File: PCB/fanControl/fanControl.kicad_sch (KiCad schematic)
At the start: 81 parts, among them J1 USB_B_Micro, J2 Barrel_Jack_Switch, J3 Conn_01x03, J4 Conn_01x06, J5 Conn_01x04, Q1 PNM723, Q2 FDD4243, Q3 BC547, Q4 PNM723, Q5 BC847BDW1, Q6 SI2324A, U1 DS18B20, U2 CH340B, U3 LM2575BT-ADJ, U4 ESP-12E, U5 LD1117S33CTR, Y1 12M

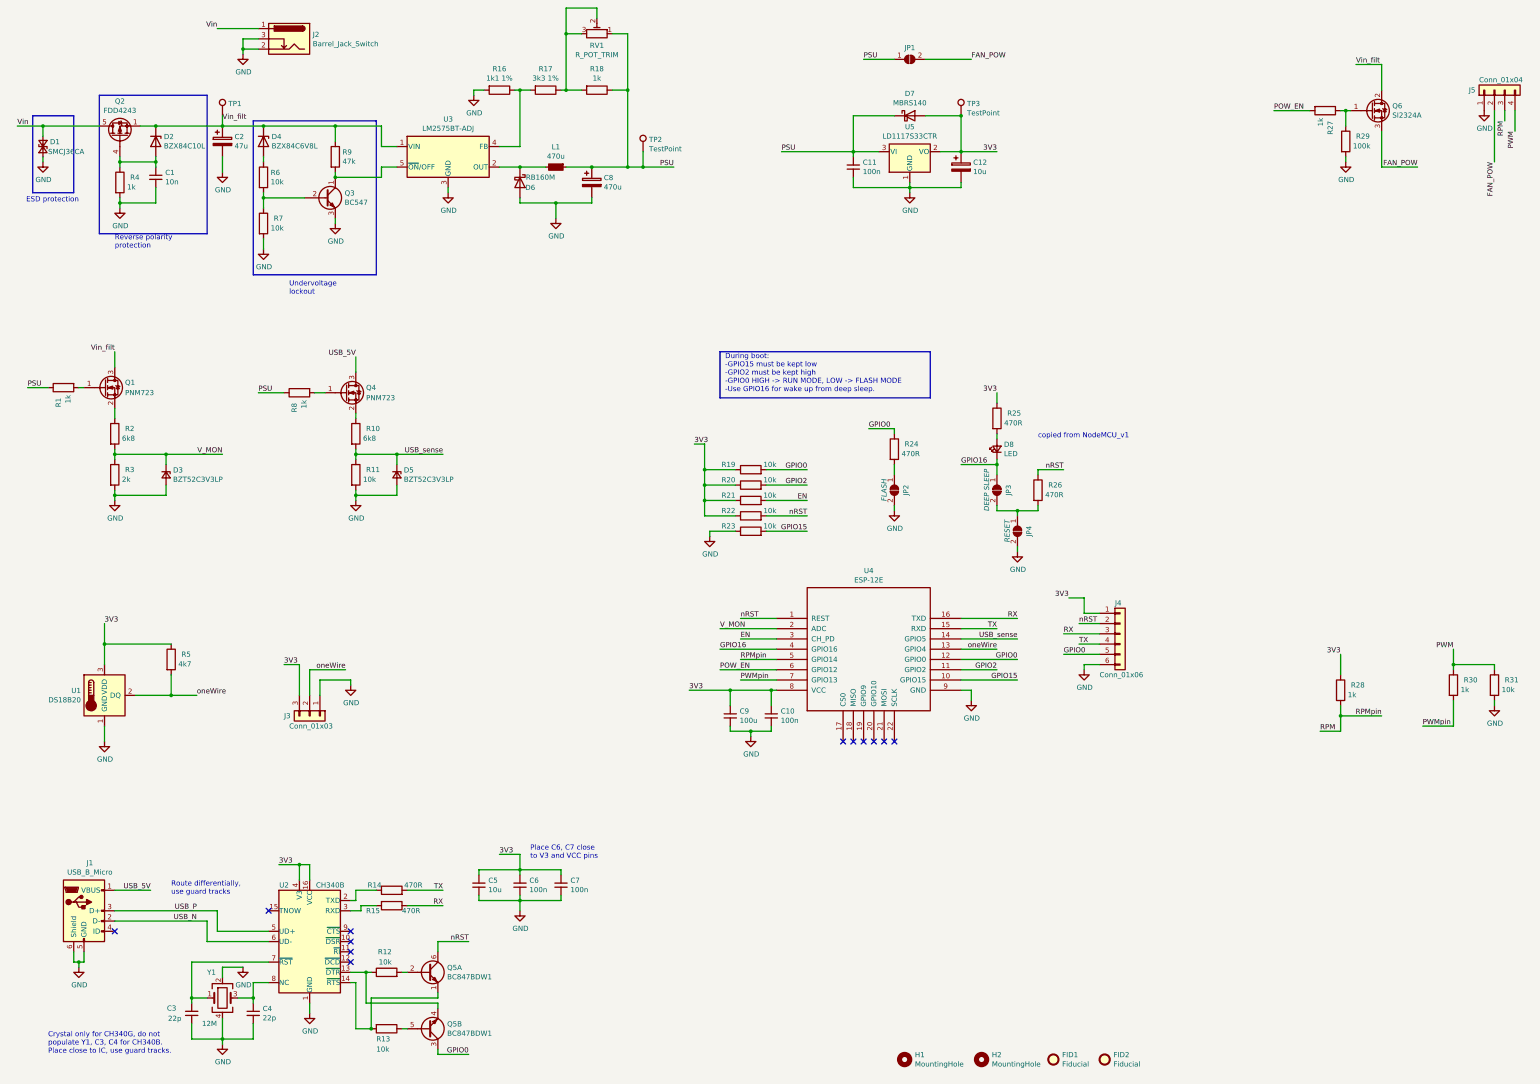
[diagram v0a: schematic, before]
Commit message: LCSC BOM done
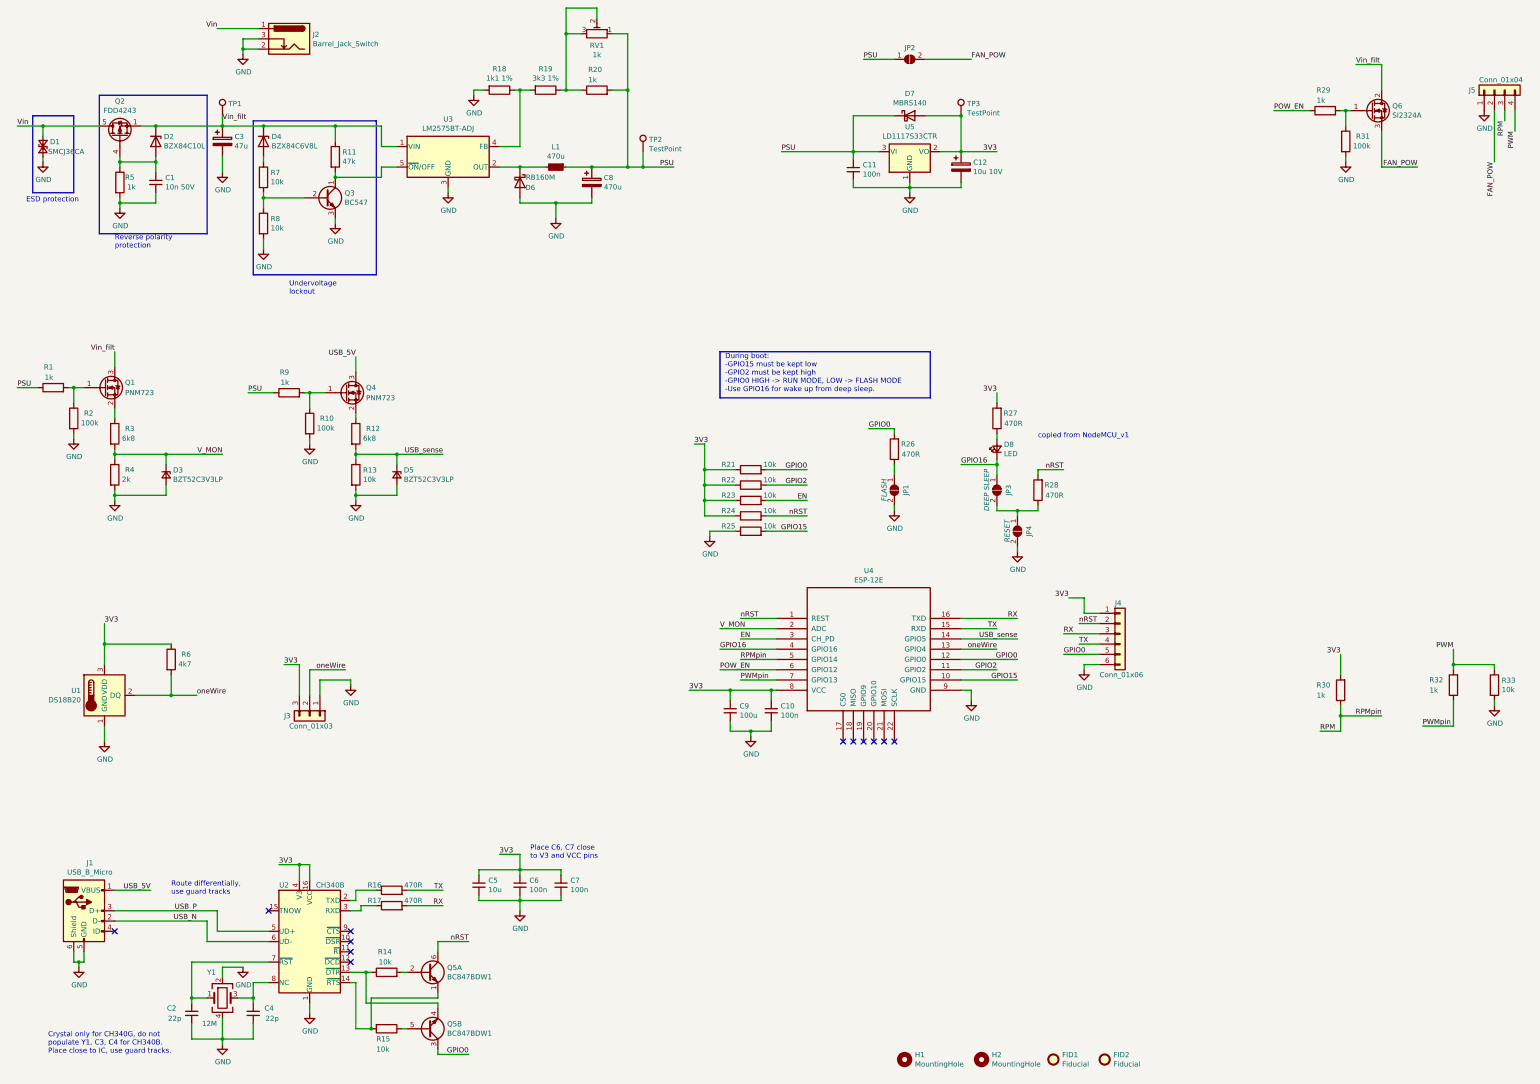
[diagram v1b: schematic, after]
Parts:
- removed R11, R19, R31, R7: 10k, agro-footprint:RES_0805, symbol Device:R
- removed R18: 1k, agro-footprint:RES_0805, symbol Device:R
- added R14, R33: 10k, agro-footprint:RES_0805, symbol Device:R
- added R17: 470R, agro-footprint:RES_0805, symbol Device:R
- added R2: 100k, agro-footprint:RES_0805, symbol Device:R
- added R29, R32, R9: 1k, agro-footprint:RES_0805, symbol Device:R
- C1: value 10n -> 10n 50V; LCSC (none) -> C527201; MPN (none) -> CC0805JKNPO9BN103; Manufacturer (none) -> Yageo
- C10, C11, C6, C7: LCSC (none) -> C520058; MPN (none) -> CC0805GRNPO9BN220; Manufacturer (none) -> Yageo
- C12: value 10u -> 10u 10V; LCSC (none) -> C696821; MPN (none) -> T529P106M010AAE200; Manufacturer Vishay -> KEMET; PartNo 293D106X9016A2TE3 -> (none)
- C2: renamed from C3; LCSC (none) -> C541515; MPN (none) -> CC0805FRNPO9BN220; Manufacturer (none) -> Yageo
- C4: LCSC (none) -> C541515; MPN (none) -> CC0805FRNPO9BN220; Manufacturer (none) -> Yageo
- C5: LCSC (none) -> C88484; MPN (none) -> CC0805ZKY5V6BB106; Manufacturer (none) -> Yageo
- C9: footprint agro-footprint:CAP_0805 -> Capacitor_SMD:C_1206_3216Metric; LCSC (none) -> C110048; MPN (none) -> CC1206MKX5R5BB107; Manufacturer (none) -> Yageo
- D2: Field6 BZX84C10LT1G -> (none); MPN (none) -> BZX84C10LT1G
- D8: LCSC (none) -> C131208; MPN (none) -> 17-215/BHC-AP1Q2/3T; Manufacturer (none) -> Everlight Elec
- J3, J4, J5, JP3, JP4, TP1, TP2, TP3: now left out of the parts list
- JP1: renamed from JP2; now left out of the parts list
- JP2: renamed from JP1; now left out of the parts list
- R1, R30: LCSC (none) -> C100046; MPN (none) -> RC0805JR-071KL; Manufacturer (none) -> Yageo
- R10: value 6k8 -> 100k; LCSC (none) -> C100049; MPN (none) -> RC0805JR-07100KL; Manufacturer (none) -> Yageo
- R11: renamed from R9; LCSC (none) -> C131051; MPN (none) -> RC0805JR-0747KL; Manufacturer (none) -> Yageo
- R12: value 10k -> 6k8; LCSC (none) -> C137409; MPN (none) -> RC0805JR-076K8L; Manufacturer (none) -> Yageo
- R13, R21, R22, R23: LCSC (none) -> C100047; MPN (none) -> RC0805JR-0710KL; Manufacturer (none) -> Yageo
- R15, R24, R25: value 470R -> 10k; LCSC (none) -> C100047; MPN (none) -> RC0805JR-0710KL; Manufacturer (none) -> Yageo
- R16: renamed from R14; LCSC (none) -> C114747; MPN (none) -> RC0805JR-07470RL; Manufacturer (none) -> Yageo
- R18: renamed from R16; LCSC (none) -> C185294; MPN (none) -> RC0805FR-071K1L; Manufacturer (none) -> Yageo
- R19: renamed from R17; LCSC (none) -> C114531; MPN (none) -> RC0805FR-073K3L; Manufacturer (none) -> Yageo
- R20: value 10k -> 1k; LCSC (none) -> C100046; MPN (none) -> RC0805JR-071KL; Manufacturer (none) -> Yageo
- R26: LCSC (none) -> C114747; MPN (none) -> RC0805JR-07470RL; Manufacturer (none) -> Yageo
- R27, R28: value 1k -> 470R; LCSC (none) -> C114747; MPN (none) -> RC0805JR-07470RL; Manufacturer (none) -> Yageo
- R3: renamed from R2; LCSC (none) -> C137409; MPN (none) -> RC0805JR-076K8L; Manufacturer (none) -> Yageo
- R31: renamed from R29; LCSC (none) -> C100049; MPN (none) -> RC0805JR-07100KL; Manufacturer (none) -> Yageo
- R4: renamed from R3; LCSC (none) -> C114748; MPN (none) -> RC0805JR-072KL; Manufacturer (none) -> Yageo
- R5: renamed from R4; LCSC (none) -> C100046; MPN (none) -> RC0805JR-071KL; Manufacturer (none) -> Yageo
- R6: renamed from R5; LCSC (none) -> C105427; MPN (none) -> RC0805JR-074K7L; Manufacturer (none) -> Yageo
- R7: renamed from R6; LCSC (none) -> C100047; MPN (none) -> RC0805JR-0710KL; Manufacturer (none) -> Yageo
- R8: value 1k -> 10k; LCSC (none) -> C100047; MPN (none) -> RC0805JR-0710KL; Manufacturer (none) -> Yageo
- RV1: value R_POT_TRIM -> 1k
- renumbered C2 to C3
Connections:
- net 3V3: now also R23.1, R24.1, R27.2, R30.2; no longer R20.1, R25.1, R28.1
- net EN: now also R23.2; no longer R21.2
- net GND: now also C4.1, R10.2, R13.2, R25.1, R8.2, R2.2, R33.2; no longer C4.2, R23.1
- net GPIO0: now also R21.2, R26.2; no longer R24.1
- net GPIO15: now also R25.2; no longer R23.2
- net GPIO2: now also R22.2; no longer R20.2
- net POW_EN: now also R29.1; no longer R27.2
- net PSU: now also R20.2, R9.1; no longer R8.1
- net PWM: now also R32.2, R33.1; no longer R30.1
- net PWMpin: now also R32.1; no longer R30.2
- net RPM: now also R30.1; no longer R28.2
- net RX: now also R17.2; no longer R15.1
- net USB_sense: now also R12.2, R13.1; no longer R10.2
- net nRST: now also R24.2, R28.2; no longer R22.2, R26.1
- net at Q3.2 (B), R7.2: now also R8.1
- net at R19.1, RV1.2, RV1.3: now also R20.1
- net at Q6.1 (G), R31.1: now also R29.2; no longer R27.1
- net at R10.1: now also Q4.1 (G), R9.2; no longer Q4.2 (S)
- net at Q1.1 (G), R1.2: now also R2.1
- net at R15.2: now also Q5.1 (E1), U2.14 (~{RTS}); no longer U2.3 (RXD)
- net at U2.8 (NC), Y1.3: now also C4.2; no longer C4.1
- net at Q5.5 (B2): now also R15.1; no longer R13.1
- net at Q5.4 (E2), U2.13 (~{DTR}): now also R14.1; no longer R12.1
- net at Q5.2 (B1): now also R14.2; no longer R12.2
- net at JP1.1 (A): now also R26.1; no longer R24.2
- net at D8.2 (A): now also R27.1; no longer R25.2
- net at JP3.2 (B), JP4.1 (A): now also R28.1; no longer R26.2
- new net: R17.1, U2.3 (RXD)
- new net: Q4.2 (S), R12.1
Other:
- moved on the sheet: C1, C9

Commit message: ver2
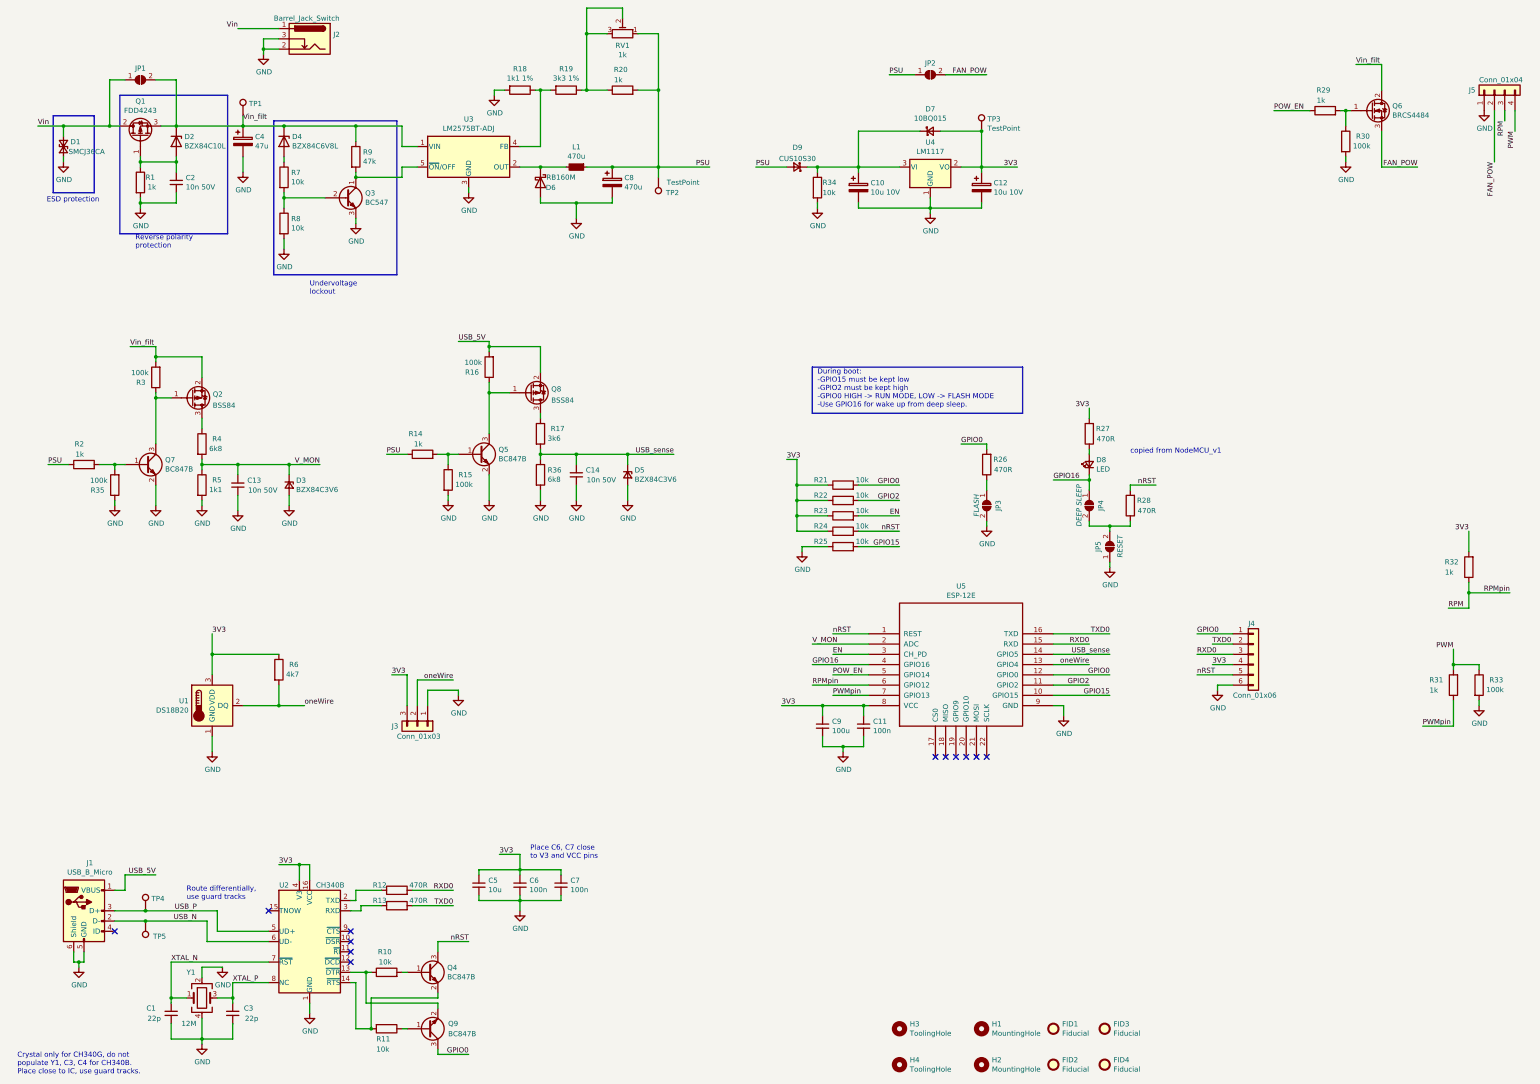
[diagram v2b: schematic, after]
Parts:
- removed C11: 100n, agro-footprint:CAP_0805, symbol agro-symbol:CAP
- removed Q1, Q4: PNM723, Package_TO_SOT_SMD:SOT-723, symbol Device:Q_NMOS_GSD
- removed Q2: FDD4243, fanControl:TO-252-2_TabPin5, symbol Transistor_FET:DMP3013SFV
- removed Q5: BC847BDW1, Package_TO_SOT_SMD:SOT-363_SC-70-6, symbol Transistor_BJT:BC847BDW1
- removed R12: 6k8, agro-footprint:RES_0805, symbol Device:R
- removed R13: 10k, agro-footprint:RES_0805, symbol Device:R
- added C10: 10u 10V, Capacitor_Tantalum_SMD:CP_EIA-3216-18_Kemet-A_Pad1.58x1.35mm_HandSolder, symbol Device:CP
- added C13, C14: 10n 50V, agro-footprint:CAP_0805, symbol agro-symbol:CAP
- added D9: CUS10S30, Diode_SMD:D_SOD-323_HandSoldering, symbol agro-symbol:SCHOTTKY
- added FID2, FID4: Fiducial, Fiducial:Fiducial_0.5mm_Mask1.5mm, symbol Mechanical:Fiducial
- added H3, H4: ToolingHole, fanControl:JLC_toolinghole, symbol Mechanical:MountingHole
- added JP1: SolderJumper_2_Open, Jumper:SolderJumper-2_P1.3mm_Open_TrianglePad1.0x1.5mm, symbol Jumper:SolderJumper_2_Open
- added Q1: FDD4243, Package_TO_SOT_SMD:TO-252-2, symbol Device:Q_PMOS_GDS
- added Q2, Q8: BSS84, Package_TO_SOT_SMD:SOT-23, symbol Device:Q_PMOS_GSD
- added Q4, Q5, Q7, Q9: BC847B, Package_TO_SOT_SMD:SOT-23, symbol Transistor_BJT:BC847
- added R16, R35: 100k, agro-footprint:RES_0805, symbol Device:R
- added R17: 3k6, agro-footprint:RES_0805, symbol Device:R
- added R34: 10k, agro-footprint:RES_0805, symbol Device:R
- added R36: 6k8, agro-footprint:RES_0805, symbol Device:R
- added TP4, TP5: TestPoint, TestPoint:TestPoint_Pad_D1.0mm, symbol Connector:TestPoint
- C1: renamed from C2; Supplier (none) -> LCSC
- C11: renamed from C10; LCSC C520058 -> C49678; MPN CC0805GRNPO9BN220 -> CC0805KRX7R9BB104; Supplier (none) -> LCSC
- C12, C5, C9, D1, D2, D4, D8, J1, R18, R19, R20, R21, R22, R23, R24, R25, R26, R27, R28, R29, R6, R7, R8, U2, U3: Supplier (none) -> LCSC
- C2: renamed from C1; Supplier (none) -> LCSC
- C3: renamed from C4; Supplier (none) -> LCSC
- C6, C7: LCSC C520058 -> C49678; MPN CC0805GRNPO9BN220 -> CC0805KRX7R9BB104; Supplier (none) -> LCSC
- D3, D5: value BZT52C3V3LP -> BZX84C3V6; footprint Package_DFN_QFN:Diodes_DFN1006-3 -> Diode_SMD:D_SOT-23_ANK; LCSC C150478 -> C94413; MPN BZT52C3V3LP-7 -> BZX84C3V6LT1G; Manufacturer Diodes Incorporated -> onsemi; Supplier (none) -> LCSC
- D6: MPN RB160MM-40TR -> RB160M-40TR; Supplier (none) -> LCSC
- D7: value MBRS140 -> 10BQ015; symbol Diode:1N5819 -> agro-symbol:SCHOTTKY; LCSC C133091 -> C413466; MPN MBRS140T3G -> VS-10BQ015-M3/5BT; Manufacturer onsemi -> Vishay; Supplier (none) -> LCSC
- FID1, H1, H2, J3, J4, J5, JP2, TP1, TP2, TP3: Supplier (none) -> NOT FITTED
- FID3: renamed from FID2; Supplier (none) -> NOT FITTED
- J2: footprint fanControl:BarrelJack_Wuerth_6941xx301002 -> Connector_BarrelJack:BarrelJack_GCT_DCJ200-10-A_Horizontal; MPN (none) -> 694106301002; Manufacturer (none) -> Wuerth
- JP3: renamed from JP1; Supplier (none) -> NOT FITTED
- JP4: renamed from JP3; Supplier (none) -> NOT FITTED
- JP5: renamed from JP4; Supplier (none) -> NOT FITTED
- Q3, U1: footprint Package_TO_SOT_THT:TO-92_Inline -> Package_TO_SOT_THT:TO-92_Inline_Wide; Supplier (none) -> LCSC; now left out of the parts list
- Q6: value SI2324A -> BRCS4484; footprint Package_TO_SOT_SMD:SOT-23 -> fanControl:BRCS4484; LCSC C779229 -> C914060; MPN SI2324A-TP -> BRCS4484SC; Manufacturer MCC -> Foshan Blue Rocket Elec; Supplier (none) -> LCSC
- R1: renamed from R5; Supplier (none) -> LCSC
- R10: renamed from R14; Supplier (none) -> LCSC
- R11: renamed from R15; Supplier (none) -> LCSC
- R12: renamed from R16; Supplier (none) -> LCSC
- R13: renamed from R17; Supplier (none) -> LCSC
- R14: renamed from R9; Supplier (none) -> LCSC
- R15: renamed from R10; Supplier (none) -> LCSC
- R2: renamed from R1; Supplier (none) -> LCSC
- R3: renamed from R2; Supplier (none) -> LCSC
- R30: renamed from R31; Supplier (none) -> LCSC
- R31: renamed from R32; Supplier (none) -> LCSC
- R32: renamed from R30; Supplier (none) -> LCSC
- R33: value 10k -> 100k; LCSC C100047 -> C100049; MPN RC0805JR-0710KL -> RC0805JR-07100KL; Supplier (none) -> LCSC
- R4: renamed from R3; LCSC C137409 -> (none); MPN RC0805JR-076K8L -> (none); Supplier (none) -> LCSC
- R5: renamed from R4; value 2k -> 1k1; LCSC C114748 -> (none); MPN RC0805JR-072KL -> (none); Supplier (none) -> LCSC
- R9: renamed from R11; Supplier (none) -> LCSC
- RV1: footprint fanControl:BournsTC42X -> fanControl:pot; Supplier (none) -> LCSC
- U4: renamed from U5; value LD1117S33CTR -> LM1117; LCSC C35879 -> C23984; MPN LD1117S33CTR -> LM1117IMPX-3.3/NOPB; Manufacturer STMicroelectronics -> Texas Instruments; Supplier (none) -> LCSC
- U5: renamed from U4; Supplier (none) -> LCSC
- Y1: footprint Crystal:Crystal_SMD_3225-4Pin_3.2x2.5mm_HandSoldering -> Crystal:Crystal_SMD_3225-4Pin_3.2x2.5mm; Supplier (none) -> LCSC
- renumbered C3 to C4
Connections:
- net 3V3: now also J4.4 (Pin_4); no longer J4.1 (Pin_1)
- net GND: now also JP5.1 (A), C10.2, C13.2, C14.2, Q5.2 (E), Q7.2 (E), R34.2, R35.1, R36.2; no longer JP5.2 (B), R3.2
- net GPIO0: now also J4.1 (Pin_1), Q9.3 (C); no longer J4.5 (Pin_5)
- net POW_EN: now also U5.5 (GPIO14); no longer U5.6 (GPIO12)
- net PSU: now also D9.2 (A); no longer D7.1 (K), U4.3 (VI)
- net RPM: now also U5.6 (GPIO12); no longer U5.5 (GPIO14)
- net USB_5V: now also Q8.2 (S), R16.2
- net USB_N: now also TP5.1
- net USB_P: now also TP4.1
- net USB_sense: now also C14.1, R17.2, R36.1
- net V_MON: now also C13.1
- net Vin: now also JP1.1 (A), Q1.2 (D)
- net Vin_filt: now also R3.2, JP1.2 (B), Q1.3 (S), Q2.2 (S)
- net nRST: now also J4.5 (Pin_5), Q4.3 (C); no longer J4.2 (Pin_2)
- net at R4.1: now also Q2.3 (D)
- net at R2.2: now also Q7.1 (B), R35.2; no longer R3.1
- net XTAL_N: now reaches C1.2, U2.7 (~{RST}), Y1.1
- net at C2.1, D2.2 (A), R1.1: now also Q1.1 (G)
- net at R11.2, U2.14 (~{RTS}): now also Q4.2 (E)
- net at R10.2: now also Q4.1 (B)
- net at R10.1, U2.13 (~{DTR}): now also Q9.2 (E)
- net at R11.1: now also Q9.1 (B)
- net at JP4.2 (B), R28.1: now also JP5.2 (B); no longer JP5.1 (A)
- net XTAL_P: now reaches C3.2, U2.8 (NC), Y1.3
- net at R14.2, R15.1: now also Q5.1 (B)
- net RX renamed TXD0
- net TXD0: now also J4.2 (Pin_2); no longer J4.3 (Pin_3)
- net TX renamed RXD0
- net RXD0: now also J4.3 (Pin_3); no longer J4.4 (Pin_4)
- new net: C10.1, D7.1 (K), D9.1 (K), R34.1, U4.3 (VI)
- new net: Q5.3 (C), Q8.1 (G), R16.1
- new net: Q2.1 (G), Q7.3 (C), R3.1
- new net: Q8.3 (D), R17.1
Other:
- moved on the sheet: C1, C11, C12, C2, C3, C4, C8, C9, D1, D2, D3, D4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
